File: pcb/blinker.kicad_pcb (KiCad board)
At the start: 2 copper layers, 55.9 x 55.9 mm, 15 parts, among them J1 ISP, U1 ATtiny10-TS

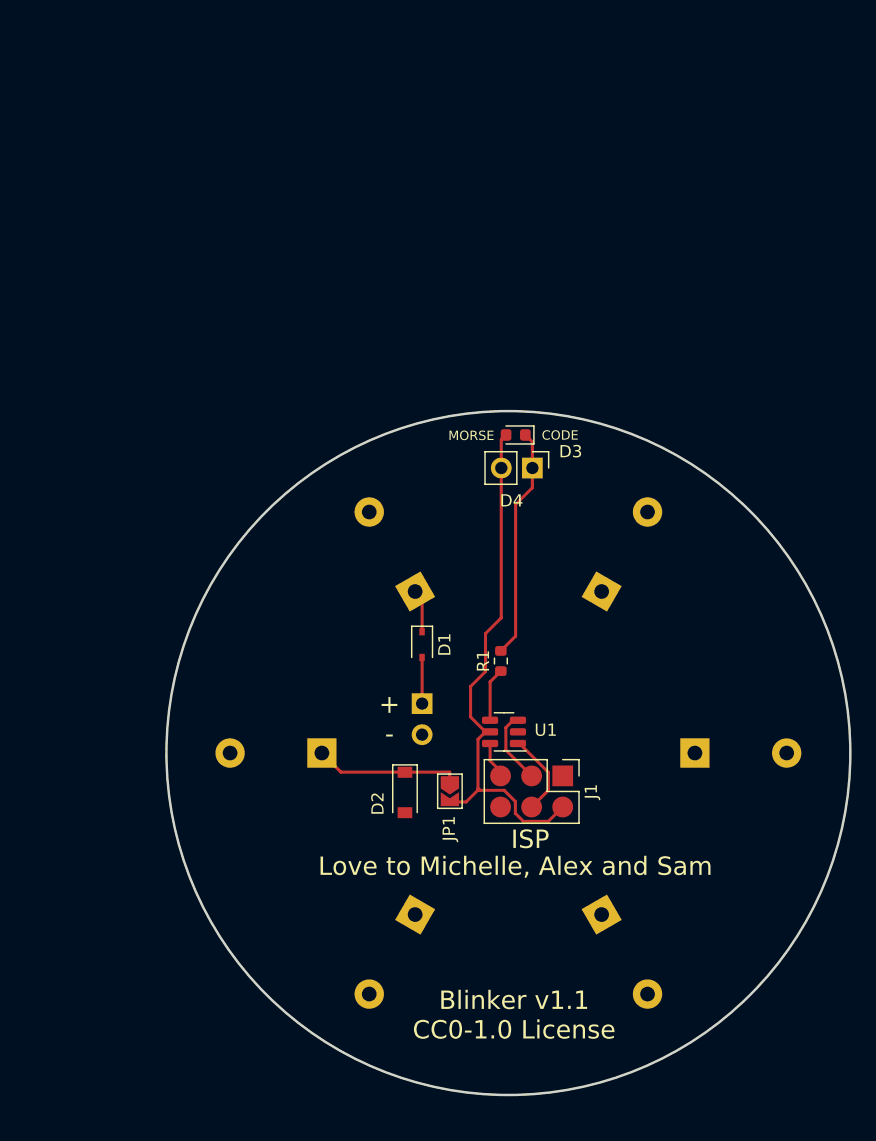
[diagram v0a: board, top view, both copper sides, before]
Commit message: v1.2 of PCB
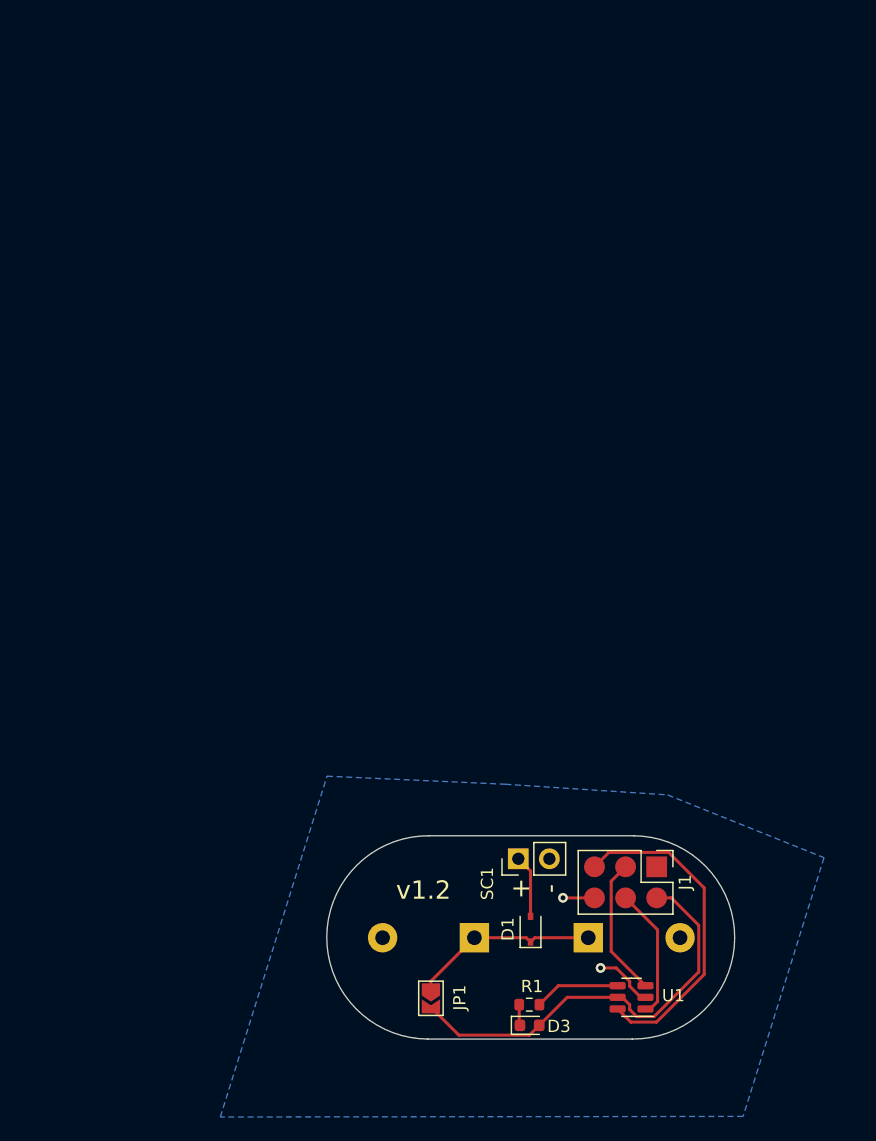
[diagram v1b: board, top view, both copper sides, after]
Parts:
- removed C3, C4, C5, C6: C_Polarized, Capacitor_THT:CP_Radial_D16.0mm_P7.50mm
- removed D2: D_Zener, Diode_SMD:D_SOD-123
- removed D4: LED, Connector_PinHeader_2.54mm:PinHeader_1x02_P2.54mm_Vertical
- SC1: moved to F.Cu
- moved D3 48.3 mm to (166.8, 123.8), turned to 0 degrees
- moved R1 28.2 mm to (166.8, 122.2), turned to 180 degrees
- moved D1 24.9 mm to (166.9, 116.0), turned to 90 degrees
- moved U1 24.1 mm to (175.2, 121.6)
- moved C1 17.4 mm to (171.6, 116.7)
- moved JP1 17.0 mm to (158.8, 121.6)
- moved SC1 14.9 mm to (165.9, 110.2), turned to 90 degrees
- moved J1 10.7 mm to (177.2, 110.9)
- moved C2 10.6 mm to (162.3, 116.7), turned to 180 degrees
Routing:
- net RESET: track 2.62 -> 26.9 mm
- net Net-(D3-Pad1): track 18.9 -> 1.71 mm
- net 5VCC: track 43.2 -> 34.7 mm
- net GND: track 0.00 -> 7.47 mm, vias 0 -> 2
- net TPICLK: track 5.67 -> 11.4 mm
- net TPIDATA: track 6.73 -> 10.8 mm
- net LED: track 4.38 -> 7.03 mm
- net /SLR_IN: track 3.77 -> 5.11 mm
- added copper zone on B.Cu, net GND
- removed copper zone on B.Cu, net 2.7VCC
- removed copper zone on F.Cu, net GND
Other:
- board size 55.9 x 55.9 mm -> 33.3 x 16.6 mm
- board text added: "v1.2"
- board text removed: "Blinker v1.1 CC0-1.0 License"
- board text removed: "CAP PWR"
- board text removed: "CODE"
- board text removed: "ISP"
- board text removed: "Love to Michelle, Alex and Sam"
- board text removed: "MORSE"
- board text removed: "SOL PNL"
